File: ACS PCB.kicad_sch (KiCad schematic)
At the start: 4 parts, among them J5 Conn_01x02

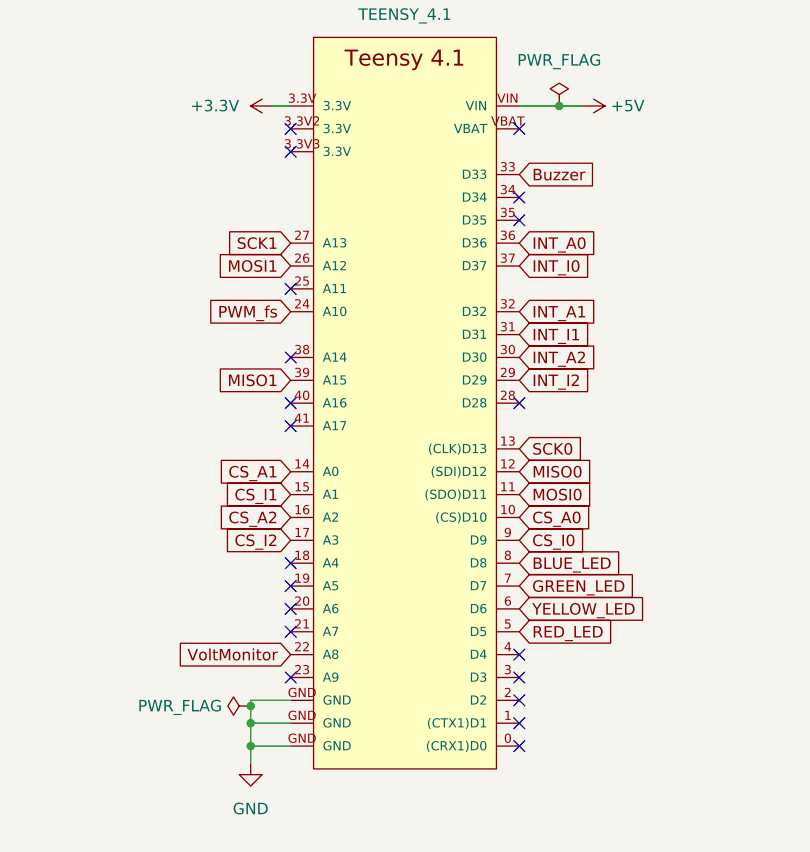
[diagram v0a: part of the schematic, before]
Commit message: Finished up PCB [DRAFT]
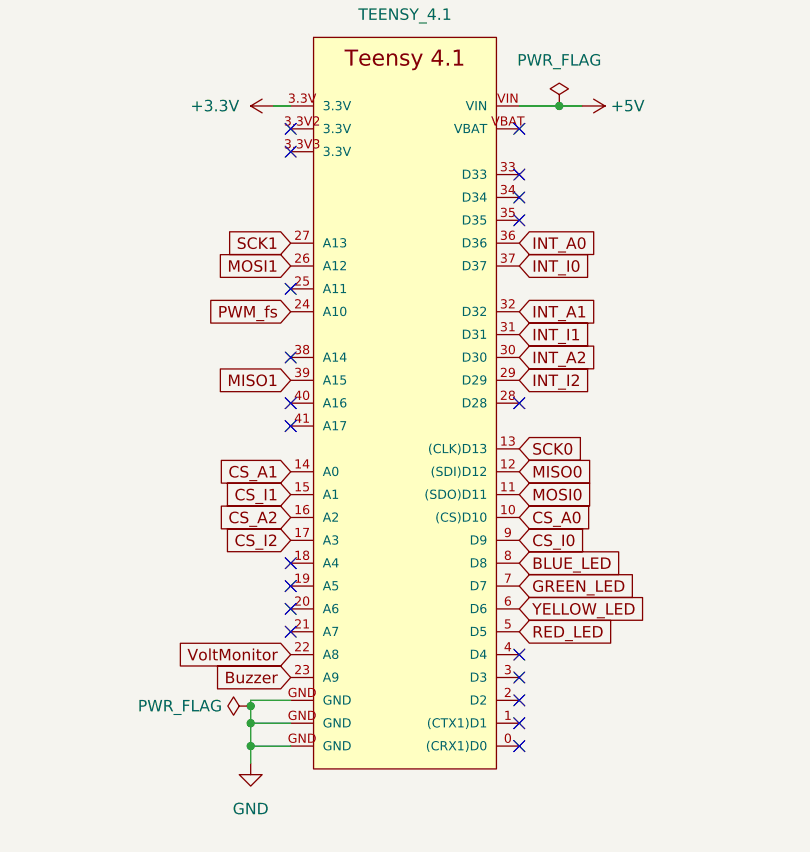
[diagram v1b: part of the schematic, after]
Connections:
- net Buzzer: now also A1.23 (A9); no longer A1.33 (D33)
